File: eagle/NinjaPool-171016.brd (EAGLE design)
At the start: 63 x 50 mm, 31 parts, among them Q1 TK13A60D, Q2 MMBT3906LT3G

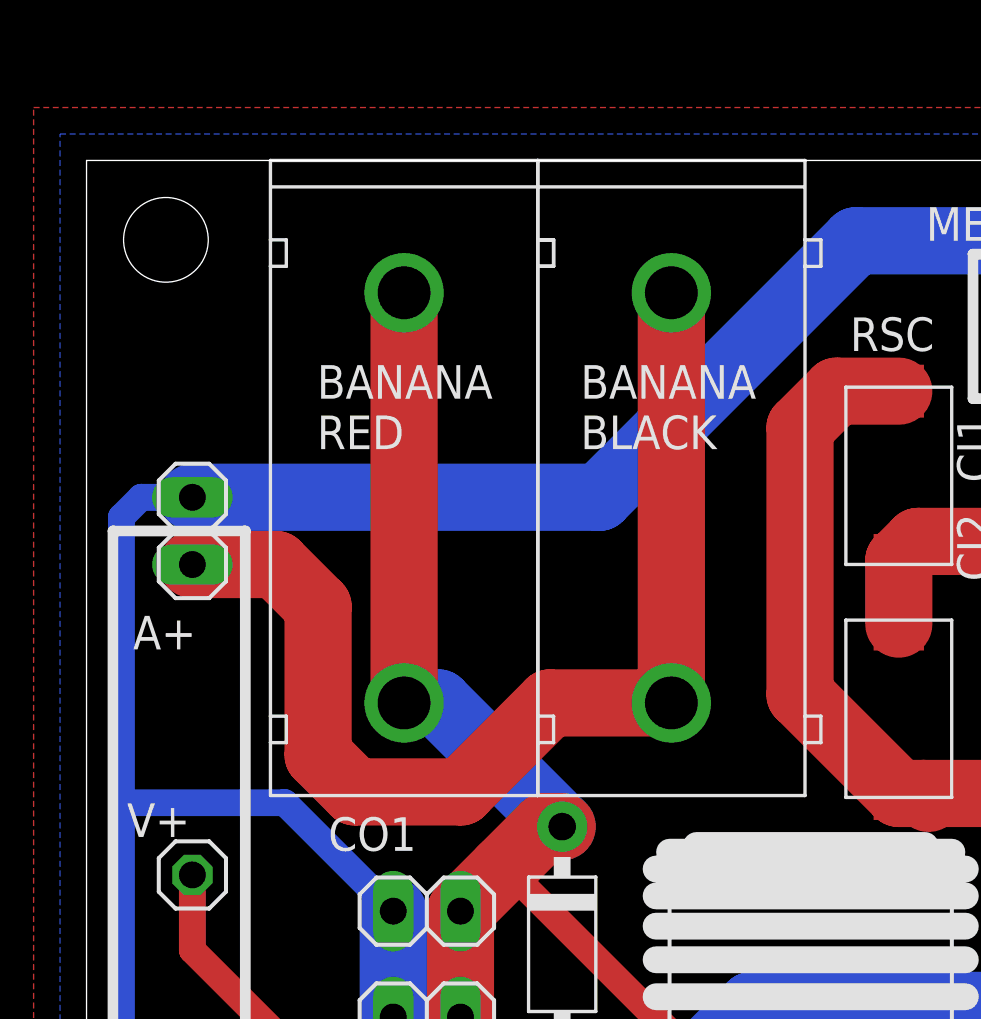
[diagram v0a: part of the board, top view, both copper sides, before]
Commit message: fixing things
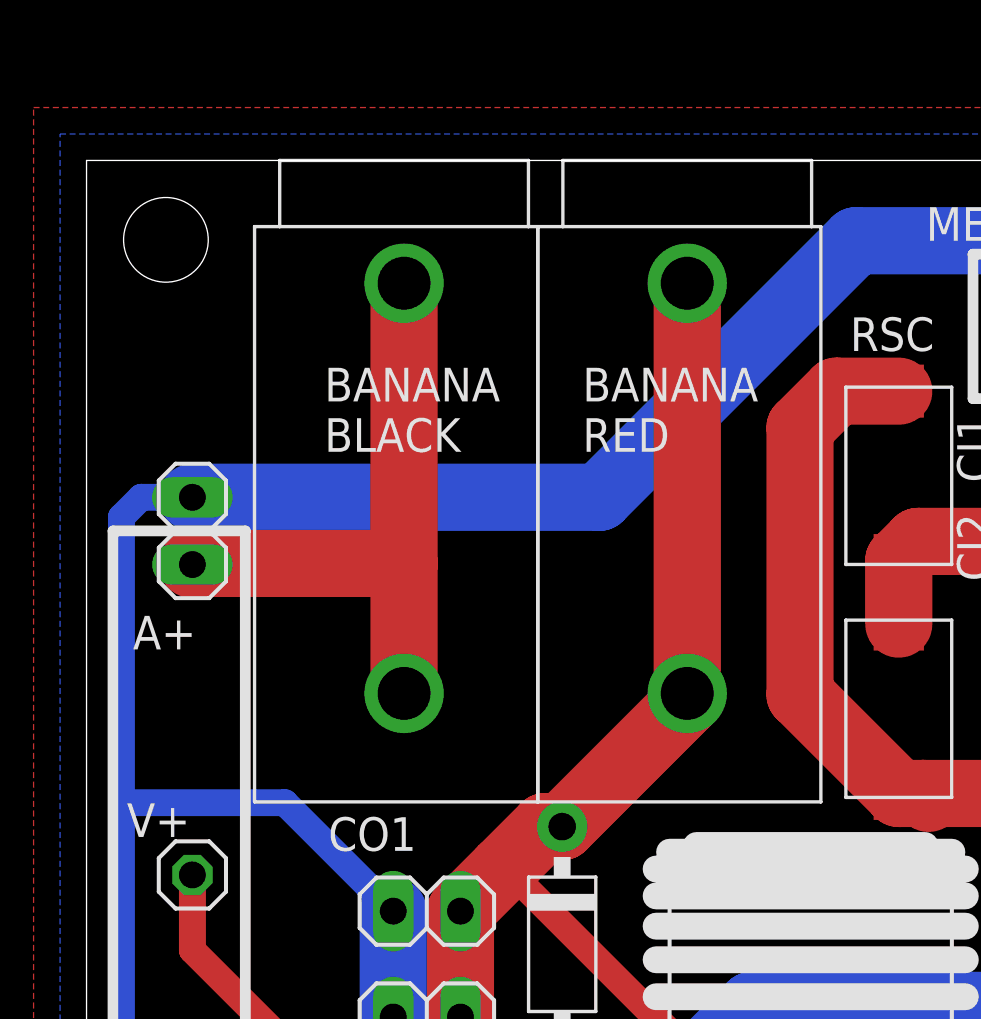
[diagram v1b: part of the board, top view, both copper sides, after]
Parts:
- removed OUT: BANANA, PCR-Connector:BANANA_TMP
- added BLACK, RED: BANANA1, PCR-Connector:BANANA
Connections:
- net A+: now also BLACK.P$1, BLACK.P$2; no longer OUT.P$3, OUT.P$4
- net VOUT: now also RED.P$1, RED.P$2; no longer OUT.P$1, OUT.P$2
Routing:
- net A+: track 41.8 -> 23.5 mm
- net VOUT: track 82.8 -> 81.8 mm
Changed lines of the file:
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@@
 <setting verticaltext="up"/>
 </settings>
-<grid distance="1" unitdist="mil" unit="mm" style="lines" multiple="1" display="yes" altdistance="0.025" altunitdist="inch" altunit="inch"/>
+<grid distance="1" unitdist="mil" unit="mil" style="lines" multiple="1" display="yes" altdistance="0.025" altunitdist="inch" altunit="inch"/>
 <layers>
 <layer number="1" name="Top" color="4" fill="1" visible="yes" active="yes"/>
@@
 <text x="1.6764" y="15.8242" size="1.27" layer="21">COM</text>
 <text x="1.7526" y="31.5214" size="1.27" layer="21">A+</text>
-<text x="8.7122" y="39.0906" size="1.27" layer="21">BANANA
+<text x="18.7452" y="38.989" size="1.27" layer="21">BANANA
 RED</text>
-<text x="18.669" y="39.0906" size="1.27" layer="21">BANANA
+<text x="8.9916" y="38.989" size="1.27" layer="21">BANANA
 BLACK</text>
 <text x="45.6184" y="6.4008" size="1.27" layer="21">TUNE</text>
@@
 </class>
 </classes>
-<designrules name="SeeedStudio_2layer_DRU_no_angle_20140221">
+<designrules name="Fusion_eagle_rule_v1.1">
 <description language="de">&lt;b&gt;EAGLE Design Rules&lt;/b&gt;
 &lt;p&gt;
@@
 </description>
 <param name="layerSetup" value="(1*16)"/>
-<param name="mtCopper" value="0.035mm 0.0175mm 0.035mm 0.035mm 0.035mm 0.035mm 0.035mm 0.035mm 0.035mm 0.035mm 0.035mm 0.035mm 0.035mm 0.035mm 0.0175mm 0.035mm"/>
-<param name="mtIsolate" value="1.5mm 1.1mm 0.2mm 0.15mm 0.2mm 0.15mm 0.2mm 0.15mm 0.2mm 0.15mm 0.2mm 0.15mm 0.2mm 0.15mm 0.2mm"/>
+<param name="mtCopper" value="0.035mm 0.035mm 0.035mm 0.035mm 0.035mm 0.035mm 0.035mm 0.035mm 0.035mm 0.035mm 0.035mm 0.035mm 0.035mm 0.035mm 0.035mm 0.035mm"/>
+<param name="mtIsolate" value="1.5mm 0.15mm 0.2mm 0.15mm 0.2mm 0.15mm 0.2mm 0.15mm 0.2mm 0.15mm 0.2mm 0.15mm 0.2mm 0.15mm 0.2mm"/>
 <param name="mdWireWire" value="6mil"/>
 <param name="mdWirePad" value="6mil"/>
@@
 </autorouter>
 <elements>
-<element name="OUT" library="PCR-Connector" package="BANANA_TMP" value="BANANA" x="12" y="50" smashed="yes" rot="R180"/>
 <element name="IC" library="PCR-IC" package="DIL8" value="MC34063/MC33063/NJM2306" x="45.4284" y="32.327" smashed="yes" rot="R90">
 <attribute name="NAME" x="44.6654" y="31.6048" size="1.27" layer="25" ratio="10"/>
@@
 <attribute name="VALUE" x="20.8534" y="3.4036" size="1.27" layer="27" rot="R90"/>
 </element>
+<element name="RED" library="PCR-Connector" package="BANANA" value="BANANA1" x="22.7" y="50" rot="R180"/>
+<element name="BLACK" library="PCR-Connector" package="BANANA" value="BANANA1" x="12" y="50" rot="R180"/>
 </elements>
 <signals>
@@
 </signal>
 <signal name="VOUT">
-<contactref element="OUT" pad="P$2"/>
-<contactref element="OUT" pad="P$1"/>
 <contactref element="CO1" pad="1"/>
 <contactref element="CO2" pad="1"/>
@@
 <contactref element="R2" pad="2"/>
 <wire x1="14.1308" y1="17.6318" x2="14.1308" y2="21.6318" width="2.54" layer="1"/>
-<wire x1="12" y1="29.5" x2="12" y2="45" width="2.54" layer="1"/>
 <contactref element="R3" pad="2"/>
 <contactref element="MODE" pad="1"/>
@@
 <wire x1="30.3784" y1="8.7376" x2="15.8964" y2="23.2196" width="1.016" layer="1"/>
 <wire x1="15.8964" y1="23.2196" x2="15.7186" y2="23.2196" width="1.016" layer="1"/>
-<wire x1="12" y1="29.5" x2="13.2992" y2="29.5" width="2.54" layer="16"/>
-<wire x1="13.2992" y1="29.5" x2="17.9748" y2="24.8244" width="2.54" layer="16"/>
 <wire x1="18.9484" y1="8.6986" x2="15.4314" y2="8.6986" width="1.016" layer="1"/>
 <wire x1="15.4314" y1="8.6986" x2="15.04" y2="9.09" width="1.016" layer="1"/>
+<contactref element="RED" pad="P$1"/>
+<contactref element="RED" pad="P$2"/>
+<wire x1="17.9748" y1="24.8244" x2="22.7" y2="29.5496" width="2.54" layer="1"/>
+<wire x1="22.7" y1="29.5496" x2="22.7" y2="29.86" width="2.54" layer="1"/>
+<wire x1="22.7" y1="29.86" x2="22.7" y2="45.36" width="2.54" layer="1"/>
 </signal>
 <signal name="N$4">
@@
 </signal>
 <signal name="A+">
-<contactref element="OUT" pad="P$3"/>
-<contactref element="OUT" pad="P$4"/>
 <contactref element="MT_A+" pad="1"/>
-<wire x1="22.1" y1="29.5" x2="22.1" y2="45" width="2.54" layer="1"/>
-<wire x1="4" y1="34.73" x2="7.167" y2="34.73" width="2.54" layer="1"/>
-<wire x1="7.167" y1="34.73" x2="8.75" y2="33.147" width="2.54" layer="1"/>
-<wire x1="8.75" y1="33.147" x2="8.75" y2="27.5336" width="2.54" layer="1"/>
-<wire x1="8.75" y1="27.5336" x2="10.147" y2="26.1366" width="2.54" layer="1"/>
-<wire x1="10.147" y1="26.1366" x2="14.1478" y2="26.1366" width="2.54" layer="1"/>
-<wire x1="14.1478" y1="26.1366" x2="17.5112" y2="29.5" width="2.54" layer="1"/>
-<wire x1="17.5112" y1="29.5" x2="22.1" y2="29.5" width="2.54" layer="1"/>
+<contactref element="BLACK" pad="P$1"/>
+<contactref element="BLACK" pad="P$2"/>
+<wire x1="12" y1="45.36" x2="12" y2="34.7726" width="2.54" layer="1"/>
+<wire x1="12" y1="34.7726" x2="12" y2="29.86" width="2.54" layer="1"/>
+<wire x1="4" y1="34.73" x2="4.0426" y2="34.7726" width="2.54" layer="1"/>
+<wire x1="4.0426" y1="34.7726" x2="12" y2="34.7726" width="2.54" layer="1"/>
 </signal>
 <signal name="N$5">
